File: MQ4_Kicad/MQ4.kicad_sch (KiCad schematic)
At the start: 4 parts, among them J1 Motor_2, J2 Motor_4, J3 Motor_1, J4 Motor_3

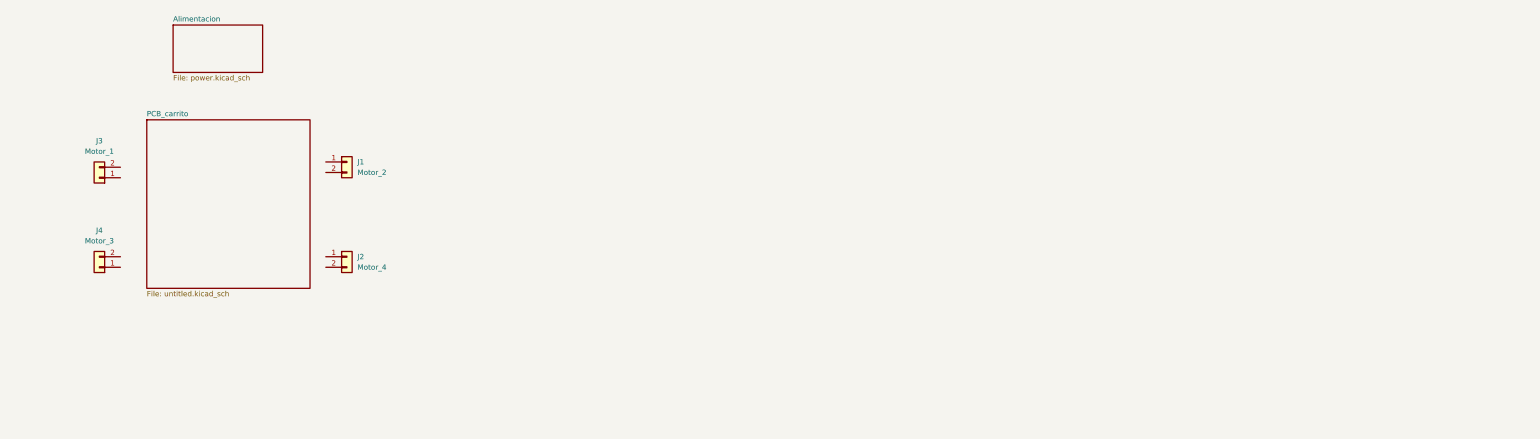
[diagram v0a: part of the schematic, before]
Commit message: Avance de esquematicos
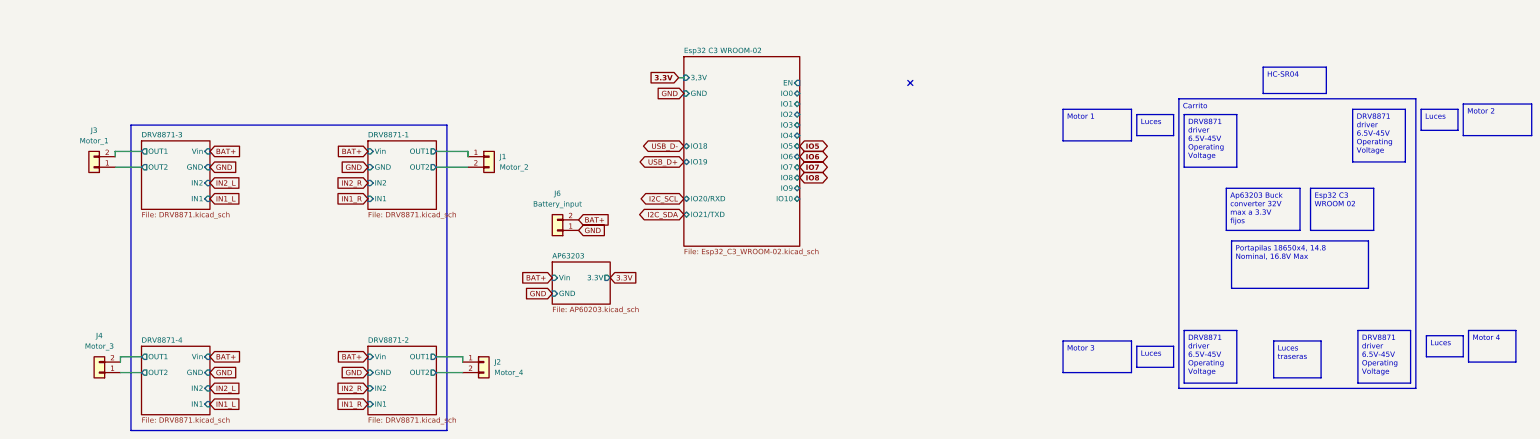
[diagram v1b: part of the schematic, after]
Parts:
- added J6: Battery_input, Connector_Molex:Molex_KK-254_AE-6410-02A_1x02_P2.54mm_Vertical, symbol Connector_Generic:Conn_01x02
- J1, J2, J3, J4: footprint (none) -> Connector_Molex:Molex_KK-254_AE-6410-02A_1x02_P2.54mm_Vertical
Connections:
- net DRV8871-3/OUT2: now reaches J3.1 (Pin_1)
- net DRV8871-3/OUT1: now reaches J3.2 (Pin_2)
- net DRV8871-4/OUT2: now reaches J4.1 (Pin_1)
- net DRV8871-4/OUT1: now reaches J4.2 (Pin_2)
- net DRV8871-1/OUT1: now reaches J1.1 (Pin_1)
- net DRV8871-1/OUT2: now reaches J1.2 (Pin_2)
- net DRV8871-2/OUT1: now reaches J2.1 (Pin_1)
- net DRV8871-2/OUT2: now reaches J2.2 (Pin_2)
- new net BAT+: J6.2 (Pin_2)
- new net GND: J6.1 (Pin_1)
- no-connect marks 0 -> 1
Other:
- removed sheet Alimentacion
- removed sheet PCB_carrito
- added sheet AP63203 (AP60203.kicad_sch)
- added sheet DRV8871-1 (DRV8871.kicad_sch)
- added sheet DRV8871-2 (DRV8871.kicad_sch)
- added sheet DRV8871-3 (DRV8871.kicad_sch)
- added sheet DRV8871-4 (DRV8871.kicad_sch)
- added sheet Esp32 C3 WROOM-02 (Esp32_C3_WROOM-02.kicad_sch)
- moved on the sheet: J1, J2, J3, J4
